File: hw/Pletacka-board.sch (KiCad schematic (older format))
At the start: 1 part

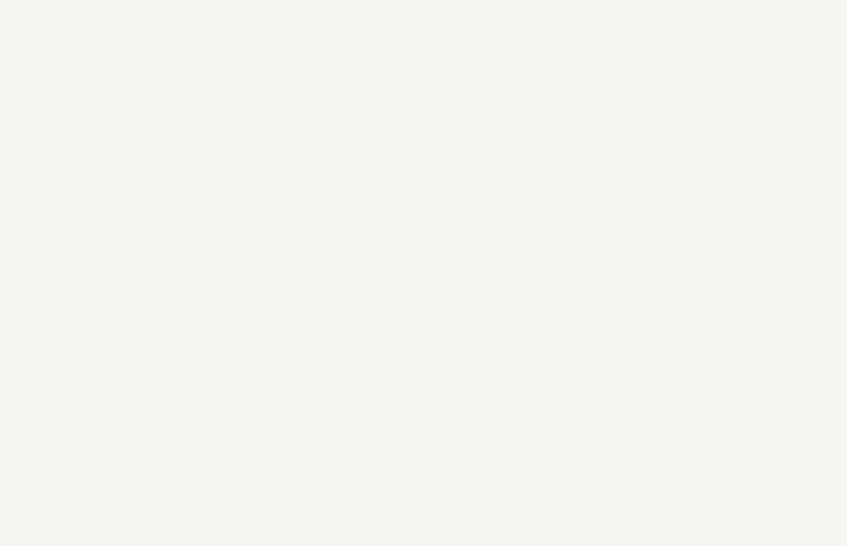
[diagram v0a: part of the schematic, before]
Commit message: Add connectors
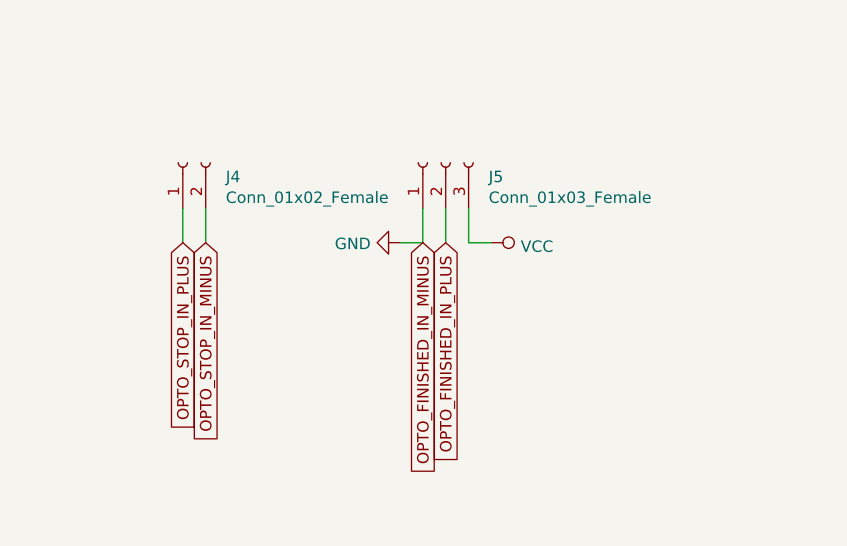
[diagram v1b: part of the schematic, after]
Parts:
- added J4: Conn_01x02_Female, Terminal_block:TerminalBlock_Phoenix_PT-1,5-2-5.0-H_1x02_P5.00mm_Horizontal, symbol Connector:Conn_01x02_Female
- added J5: Conn_01x03_Female, Terminal_block:TerminalBlock_Phoenix_PT-1,5-3-5.0-H_1x03_P5.00mm_Horizontal, symbol Connector:Conn_01x03_Female
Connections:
- net labels added: OPTO_FINISHED_IN_MINUS, OPTO_FINISHED_IN_PLUS, OPTO_STOP_IN_MINUS, OPTO_STOP_IN_PLUS, VCC
- wire segments 25 -> 32
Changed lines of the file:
@@
 F1 "Power.sch" 50
 $EndSheet
+$Comp
+L Connector:Conn_01x02_Female J4
+U 1 1 5F9151EB
+P 2550 5600
+F 0 "J4" V 2488 5412 50  0000 R CNN
+F 1 "Conn_01x02_Female" V 2397 5412 50  0000 R CNN
+F 2 "Terminal_block:TerminalBlock_Phoenix_PT-1,5-2-5.0-H_1x02_P5.00mm_Horizontal" H 2550 5600 50  0001 C CNN
+F 3 "~" H 2550 5600 50  0001 C CNN
+	1    2550 5600
+	0    -1   -1   0
+$EndComp
+$Comp
+L Connector:Conn_01x03_Female J5
+U 1 1 5F915FED
+P 3700 5600
+F 0 "J5" V 3638 5412 50  0000 R CNN
+F 1 "Conn_01x03_Female" V 3547 5412 50  0000 R CNN
+F 2 "Terminal_block:TerminalBlock_Phoenix_PT-1,5-3-5.0-H_1x03_P5.00mm_Horizontal" H 3700 5600 50  0001 C CNN
+F 3 "~" H 3700 5600 50  0001 C CNN
+	1    3700 5600
+	0    -1   -1   0
+$EndComp
+Wire Wire Line
+	2550 5950 2550 5800
+Wire Wire Line
+	2650 5950 2650 5800
+Wire Wire Line
+	3600 5950 3600 5800
+Wire Wire Line
+	3700 5950 3700 5800
+Wire Wire Line
+	3800 5950 3800 5800
+Text GLabel 2550 5950 3    50   Input ~ 0
+OPTO_STOP_IN_PLUS
+Text GLabel 2650 5950 3    50   Input ~ 0
+OPTO_STOP_IN_MINUS
+Text GLabel 3600 5950 3    50   Input ~ 0
+OPTO_FINISHED_IN_MINUS
+Text GLabel 3700 5950 3    50   Input ~ 0
+OPTO_FINISHED_IN_PLUS
+Wire Wire Line
+	3800 5950 3900 5950
+Wire Wire Line
+	3600 5950 3500 5950
+$Comp
+L power:GND #PWR0116
+U 1 1 5F91B916
+P 3500 5950
+F 0 "#PWR0116" H 3500 5700 50  0001 C CNN
+F 1 "GND" V 3505 5822 50  0000 R CNN
+F 2 "" H 3500 5950 50  0001 C CNN
+F 3 "" H 3500 5950 50  0001 C CNN
+	1    3500 5950
+	0    1    1    0
+$EndComp
+$Comp
+L power:VCC #PWR0117
+U 1 1 5F91BD5C
+P 3900 5950
+F 0 "#PWR0117" H 3900 5800 50  0001 C CNN
+F 1 "VCC" V 3917 6078 50  0000 L CNN
+F 2 "" H 3900 5950 50  0001 C CNN
+F 3 "" H 3900 5950 50  0001 C CNN
+	1    3900 5950
+	0    1    1    0
+$EndComp
 $EndSCHEMATC
